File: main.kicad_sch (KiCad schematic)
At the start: 0 parts

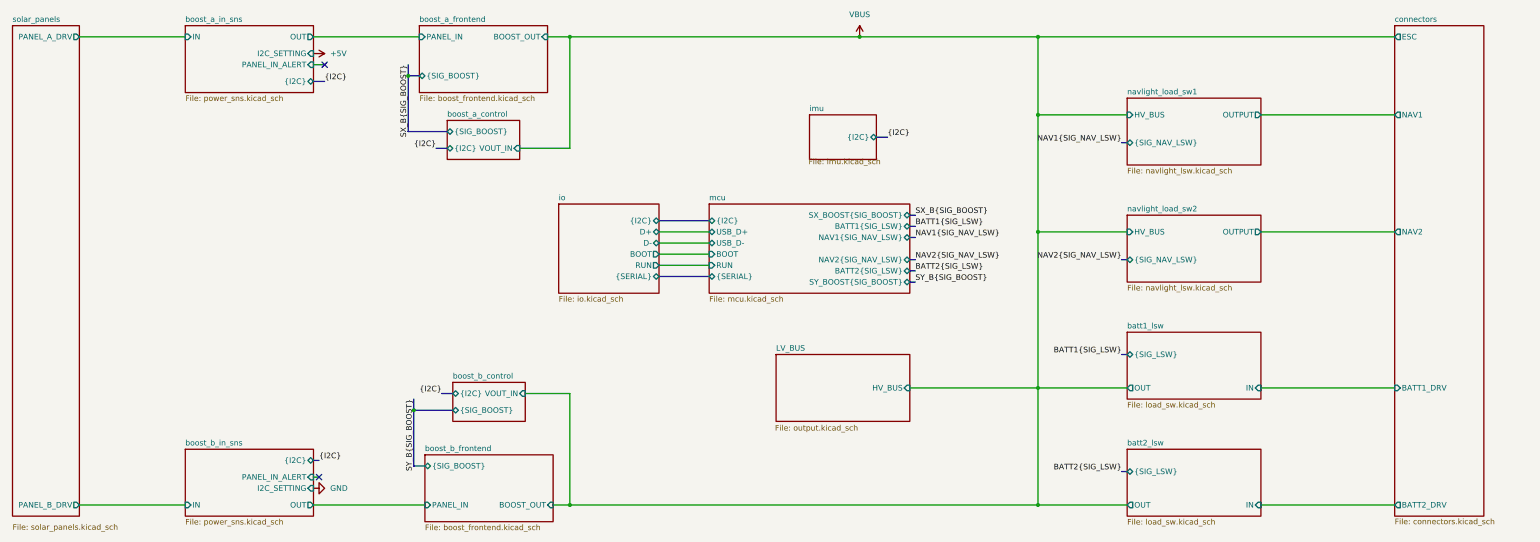
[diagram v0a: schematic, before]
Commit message: Pushing
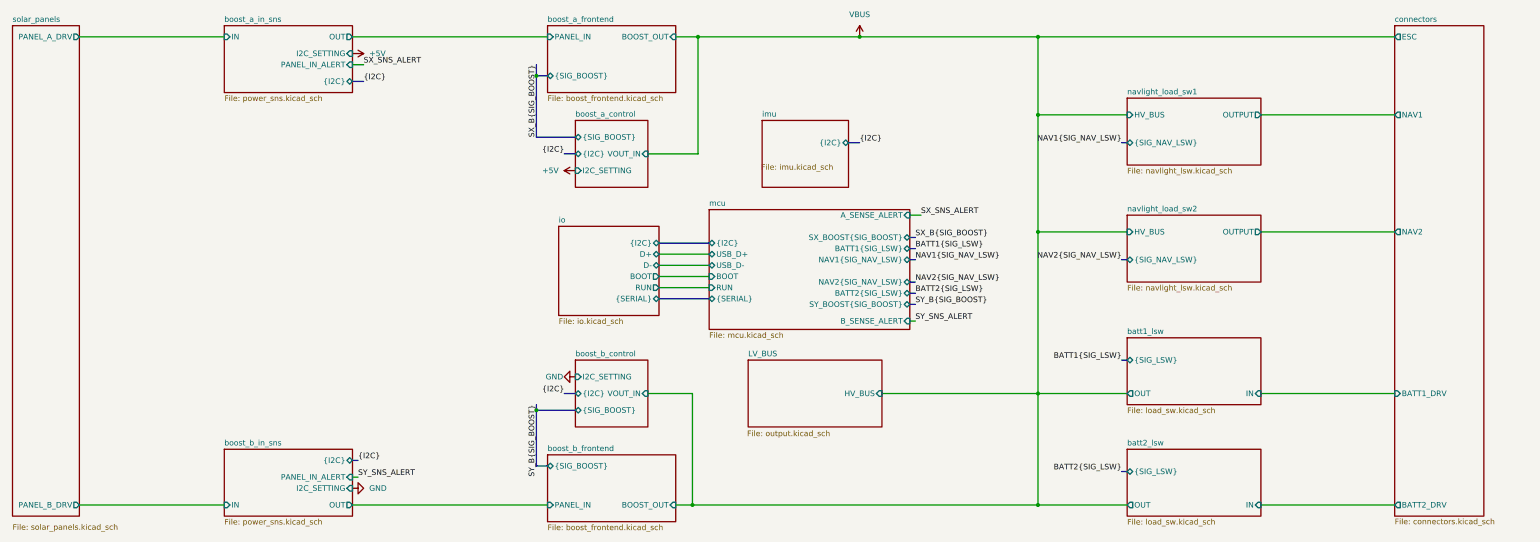
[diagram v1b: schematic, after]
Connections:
- no-connect marks 2 -> 0
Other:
- sheet boost_a_control ports: added I2C_SETTING; removed none
- sheet boost_b_control ports: added I2C_SETTING; removed none
- sheet mcu ports: added A_SENSE_ALERT, B_SENSE_ALERT; removed none
